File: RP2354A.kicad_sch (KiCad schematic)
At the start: 28 parts, among them SW1 Button, SW2 Button, U1 RP2350A, U2 ABM8-272-T3, U8 W25Q16JVUXIQ

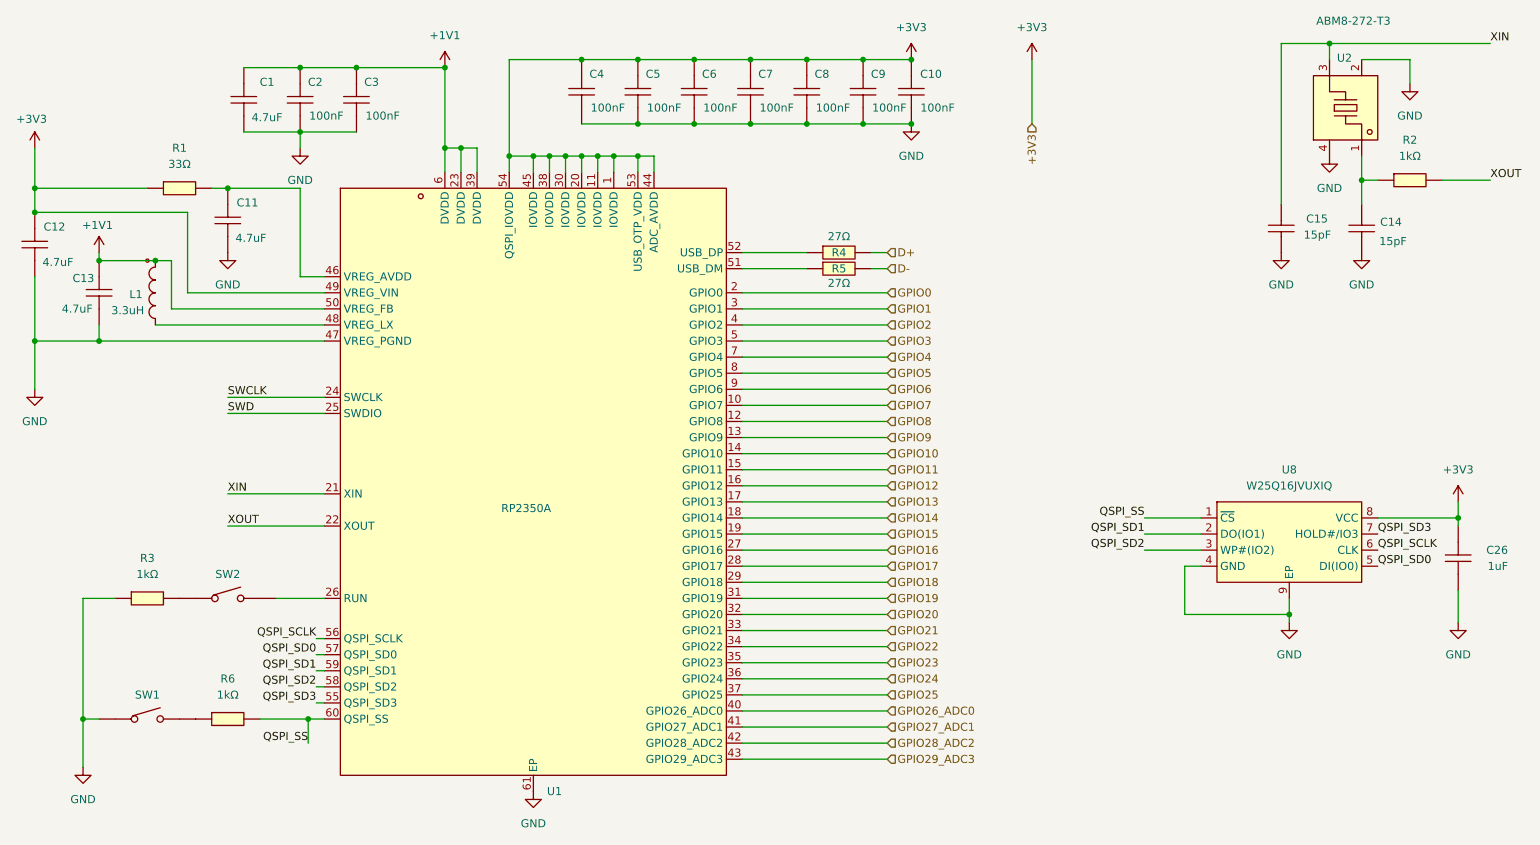
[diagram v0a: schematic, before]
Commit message: Final manufactured version
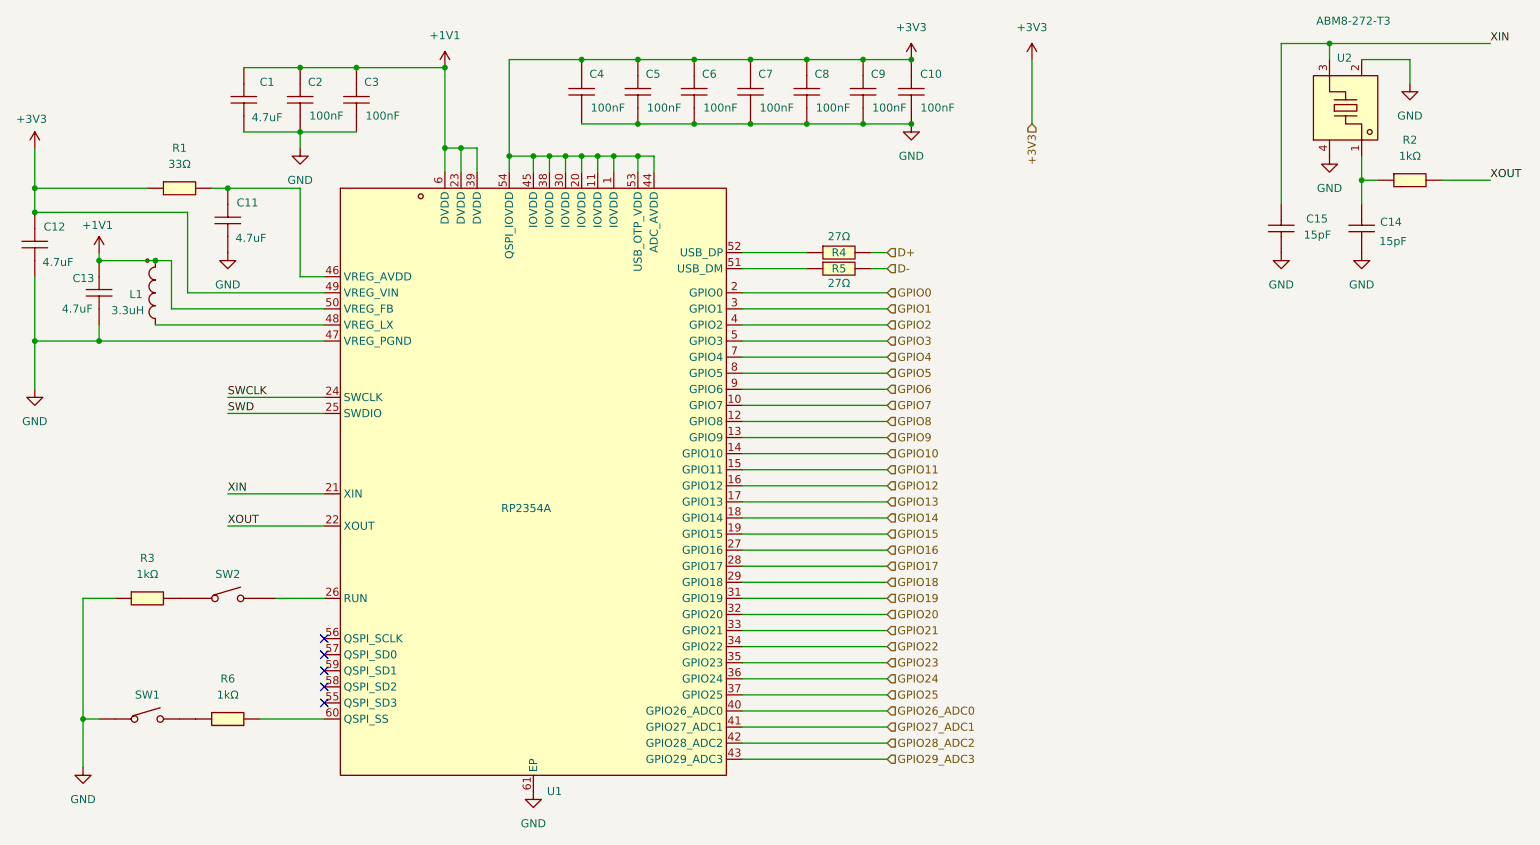
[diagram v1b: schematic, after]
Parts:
- removed C26: 1uF, Capacitors:C0402, symbol Capacitors:1uF_C0402
- removed U8: W25Q16JVUXIQ, Other:USON-8_L3.0-W2.0-P0.50-BL-EP, symbol Other:W25Q16JVUXIQ
- U1: value RP2350A -> RP2354A; LCSC Part C42411118 -> C41378174
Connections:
- net QSPI_SCLK: no longer names the net of U1.56 (QSPI_SCLK)
- net QSPI_SD0: no longer names the net of U1.57 (QSPI_SD0)
- net QSPI_SD1: no longer names the net of U1.59 (QSPI_SD1)
- net QSPI_SD2: no longer names the net of U1.58 (QSPI_SD2)
- net QSPI_SD3: no longer names the net of U1.55 (QSPI_SD3)
- net QSPI_SS: no longer names the net of R6.2, U1.60 (QSPI_SS)
- no-connect marks 0 -> 5
